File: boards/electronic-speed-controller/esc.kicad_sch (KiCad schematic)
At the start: 34 parts, among them J101 XT60PW-M, J102 39303037, U101 LMR51420XDDCR, U102 Teensy4.1

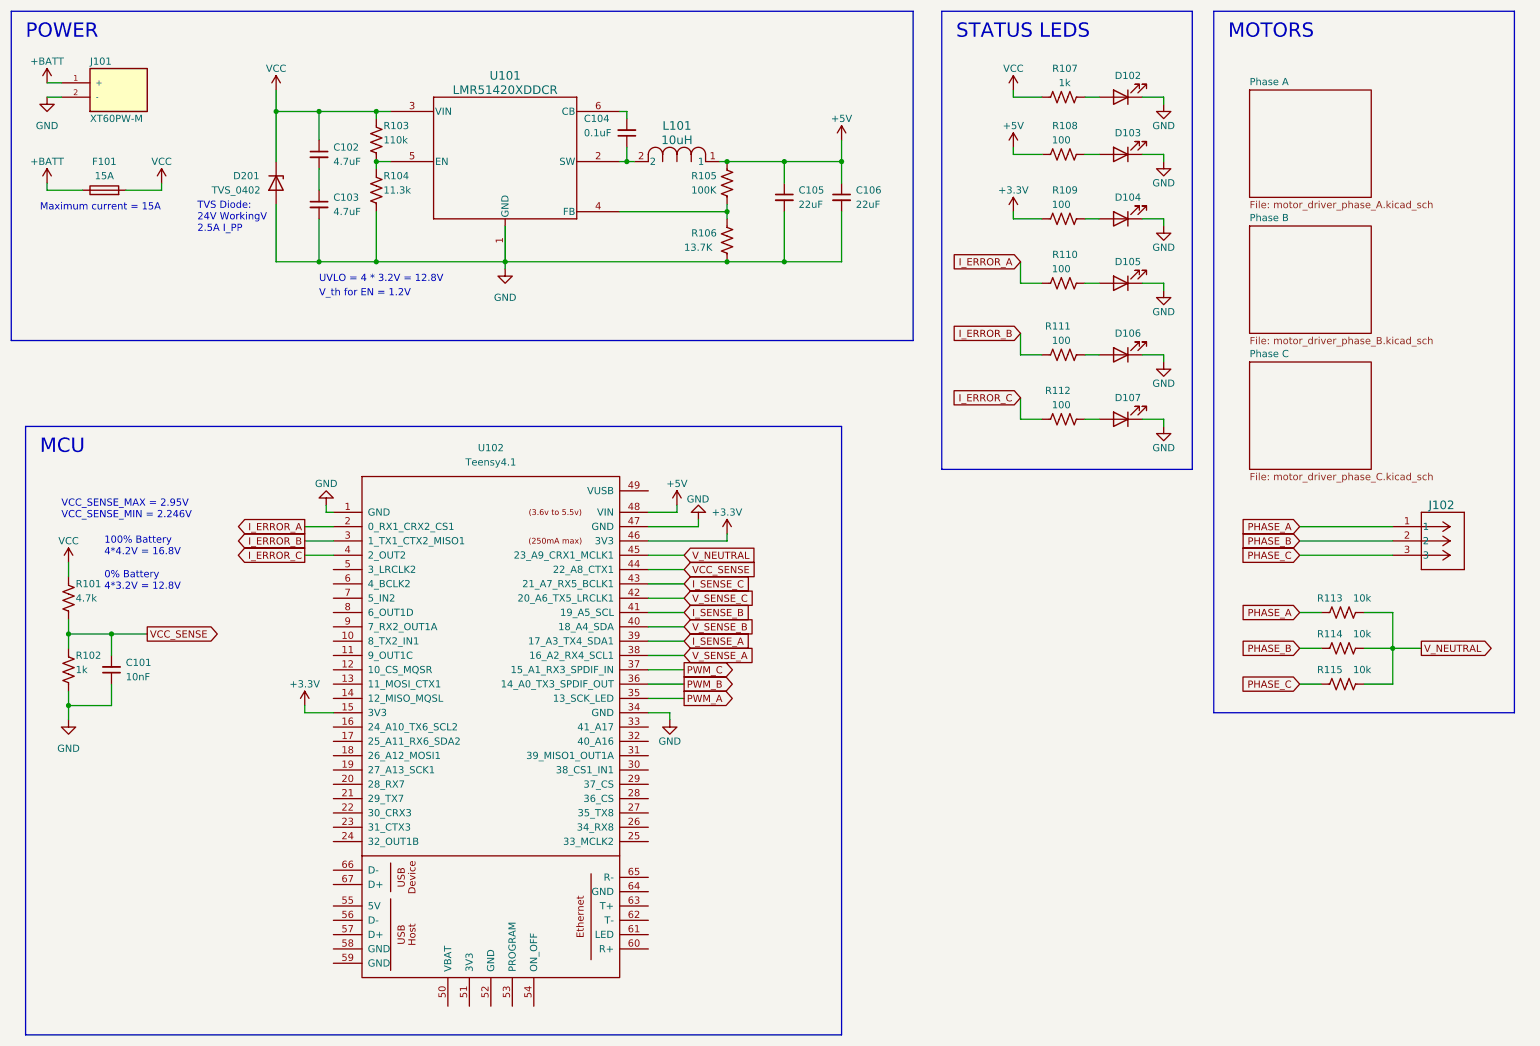
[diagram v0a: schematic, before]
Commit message: finished layout and schematic
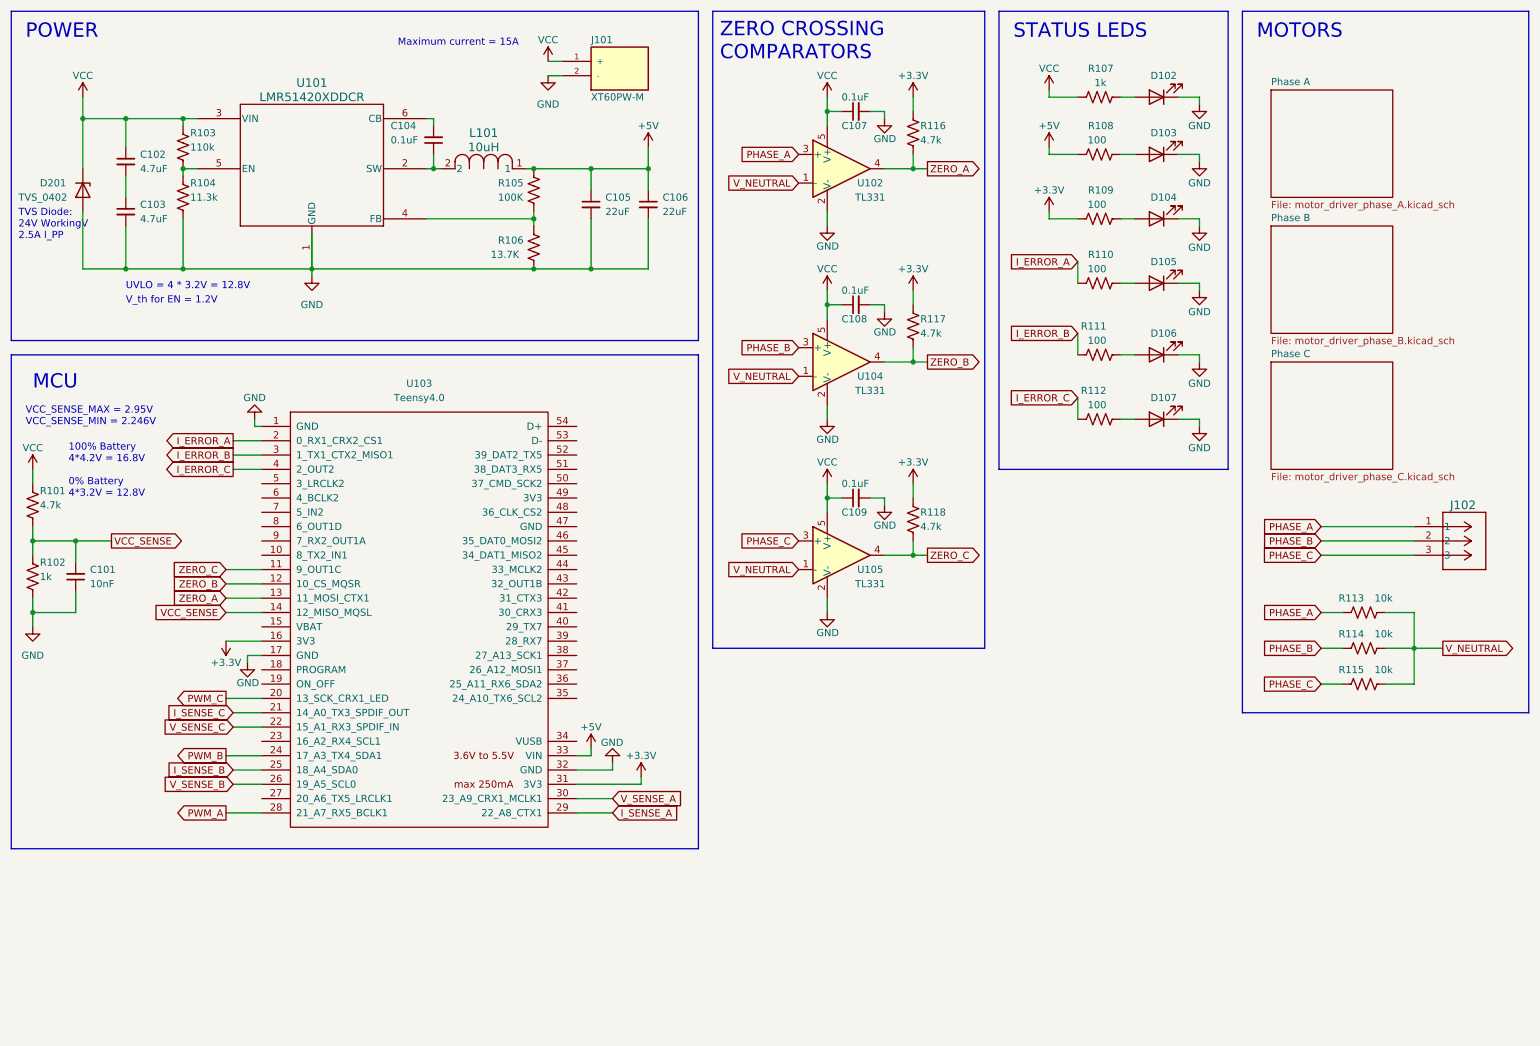
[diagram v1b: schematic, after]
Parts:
- removed F101: 15A, Fuse:Fuse_1206_3216Metric, symbol Device:Fuse
- removed U102: Teensy4.1, teensy.pretty-master:Teensy41, symbol teensy:Teensy4.1
- added C107, C108, C109: 0.1uF, Capacitor_SMD:C_0603_1608Metric, symbol Device:C_Small
- added R116, R117, R118: 4.7k, Resistor_SMD:R_0603_1608Metric, symbol Device:R_US
- added U102, U104, U105: TL331, Package_TO_SOT_SMD:SOT-23-5, symbol Comparator:TL331
- added U103: Teensy4.0, teensy.pretty-master:Teensy40, symbol teensy:Teensy4.0
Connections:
- net +BATT is gone; now on net VCC: J101.1 (+)
- net +3.3V: now also R116.1, R117.1, R118.1, U103.16 (3V3), U103.31 (3V3)
- net +5V: now also U103.33 (VIN)
- net GND: now also C107.2, C108.2, C109.2, U102.2 (V-), U103.1 (GND), U103.17 (GND), U103.32 (GND), U104.2 (V-), U105.2 (V-)
- net I_ERROR_A: now also U103.2 (0_RX1_CRX2_CS1)
- net I_ERROR_B: now also U103.3 (1_TX1_CTX2_MISO1)
- net I_ERROR_C: now also U103.4 (2_OUT2)
- net I_SENSE_A: now also U103.29 (22_A8_CTX1)
- net I_SENSE_B: now also U103.25 (18_A4_SDA0)
- net I_SENSE_C: now also U103.21 (14_A0_TX3_SPDIF_OUT)
- net PHASE_A: now also U102.3 (+)
- net PHASE_B: now also U104.3 (+)
- net PHASE_C: now also U105.3 (+)
- net PWM_A: now also U103.28 (21_A7_RX5_BCLK1)
- net PWM_B: now also U103.24 (17_A3_TX4_SDA1)
- net PWM_C: now also U103.20 (13_SCK_CRX1_LED)
- net VCC: now also C107.1, C108.1, C109.1, U102.5 (V+), U104.5 (V+), U105.5 (V+)
- net VCC_SENSE: now also U103.14 (12_MISO_MQSL)
- net V_NEUTRAL: now also U102.1 (-), U104.1 (-), U105.1 (-)
- net V_SENSE_A: now also U103.30 (23_A9_CRX1_MCLK1)
- net V_SENSE_B: now also U103.26 (19_A5_SCL0)
- net V_SENSE_C: now also U103.22 (15_A1_RX3_SPDIF_IN)
- new net ZERO_A: R116.2, U102.4, U103.13 (11_MOSI_CTX1)
- new net ZERO_B: R117.2, U103.12 (10_CS_MQSR), U104.4
- new net ZERO_C: R118.2, U103.11 (9_OUT1C), U105.4
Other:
- note added: "ZERO CROSSING COMPARATORS"
- moved on the sheet: C101, C102, C103, C104, C105, C106, D102, D103, D104, D105, D106, D107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
